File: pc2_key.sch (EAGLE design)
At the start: 25 parts, among them IC1 4011D, IC2 MC34063AD

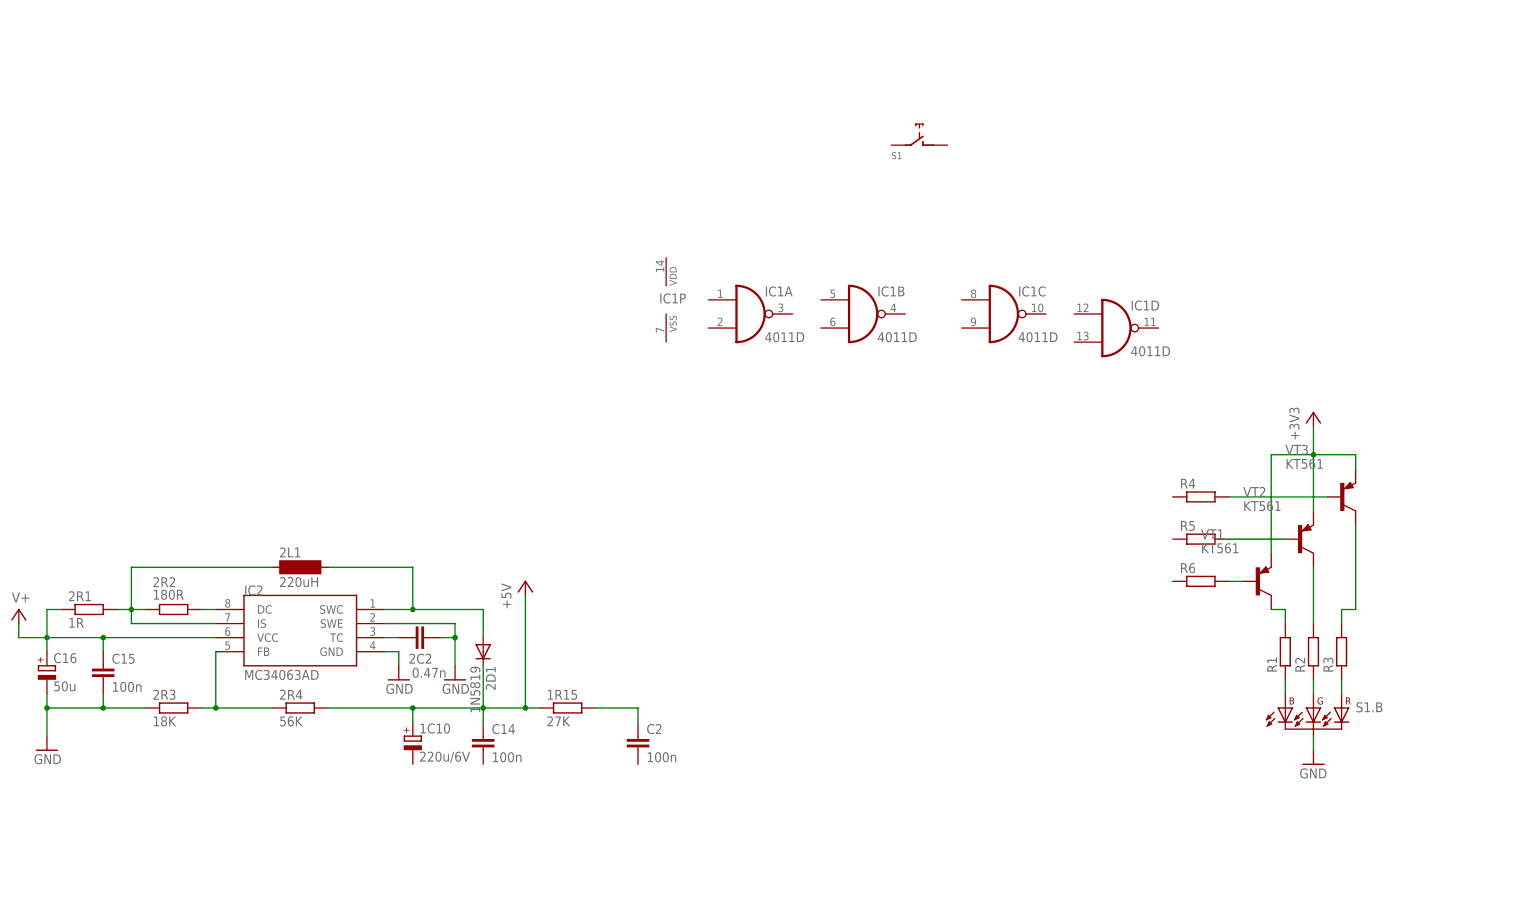
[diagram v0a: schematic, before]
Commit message: 2
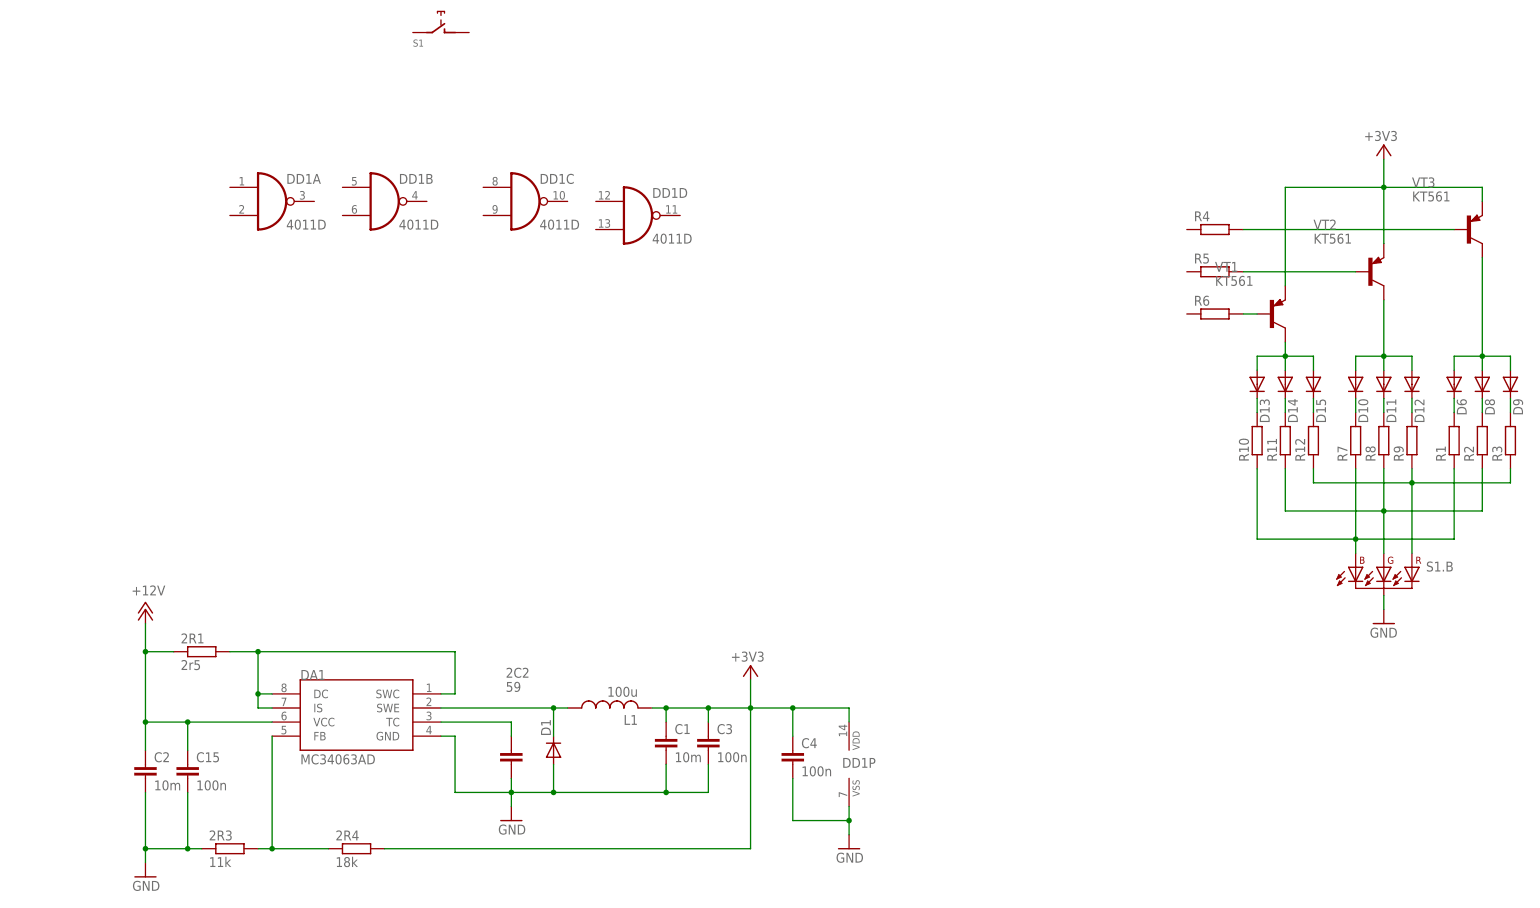
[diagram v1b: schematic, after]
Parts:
- removed 1C10: 220u/6V, resistor:CPOL-EUE3.5-8
- removed 1R15: 27K, resistor:R-EU_R0805
- removed 2D1: 1N5819, diode:DIODE-DO41-10
- removed 2L1: 220uH, inductor-neosid:SD12-1000
- removed 2R2: 180R, resistor:R-EU_R0805
- removed C14: 100n, resistor:C-EUC0805K
- removed C16: 50u, resistor:CPOL-EUE2.5-6
- removed IC1: 4011D, 40xx:4011D
- removed IC2: MC34063AD, mc34063:MC34063AD
- added C1: 10m, rcl:C-EUC1210
- added C3, C4: 100n, resistor:C-EUC0805K
- added D1: (no value), diode:DIODE-SMB
- added D10, D11, D12, D13, D14, D15, D6, D8, D9: (no value), diode:DIODE-SOD80C
- added DA1: MC34063AD, mc34063:MC34063AD
- added DD1: 4011D, 40xx:4011D
- added L1: 100u, rcl:L-US6000-XXX-RC
- added R10, R11, R12, R7, R8, R9: (no value), rcl:R-EU_R0805
- 2C2: value 0.47n -> 59
- 2R1: value 1R -> 2r5
- 2R3: value 18K -> 11k
- 2R4: value 56K -> 18k
- C2: value 100n -> 10m; device resistor:C-EUC0805K -> rcl:C-EUC1210
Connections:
- removed net +5V: 1C10.+, 1R15.1, 2D1.C, 2R4.2, C14.1
- removed net N$11: 1R15.2, C2.1
- removed net N$21: 2D1.A, 2L1.2, IC2.SWC
- removed net N$22: 2R2.2, IC2.DC
- removed net N$24: 2L1.1, 2R1.2, 2R2.1, IC2.IS
- removed net V+: 2R1.1, C15.1, C16.+, IC2.VCC
- new net +12V: 2R1.1, C15.1, C2.1, DA1.VCC
- new net N$13: R11.1, R2.1, R8.1, S1.B.G
- new net N$14: R12.1, R3.1, R9.1, S1.B.R
- new net N$15: D12.C, R9.2
- new net N$16: D11.C, R8.2
- new net N$17: D10.C, R7.2
- new net N$18: D15.C, R12.2
- new net N$20: D14.C, R11.2
- new net N$23: D13.C, R10.2
- new net N$26: D13.A, D14.A, D15.A, VT1.C
- new net N$27: D10.A, D11.A, D12.A, VT2.C
- new net N$28: D6.A, D8.A, D9.A, VT3.C
- net +3V3: now also 2R4.2, C1.1, C3.1, C4.1, DD1P.VDD, L1.2
- net GND: now also C1.2, C2.2, C3.2, C4.2, D1.A, DA1.GND, DD1P.VSS; no longer C16.-, IC2.GND, IC2.SWE
- net N$19: now also D1.C, DA1.SWE, L1.1; no longer 2C2.1, IC2.TC
- net N$25: now also DA1.FB; no longer IC2.FB
- net N$3: now also 2R1.2, DA1.DC, DA1.IS, DA1.SWC; no longer R1.2, VT1.C
- net N$4: now also R1.1, R10.1, R7.1, S1.B.B; no longer R2.2, VT2.C
- net N$5: now also 2C2.1, DA1.TC; no longer R3.2, VT3.C
- net N$6: now also D9.C, R3.2; no longer R1.1, S1.B.B
- net N$7: now also D8.C, R2.2; no longer R2.1, S1.B.G
- net N$8: now also D6.C, R1.2; no longer R3.1, S1.B.R
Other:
- moved on the sheet: 2C2, 2R1, 2R3, 2R4, C15, C2, R1, R2, R3, R4, R5, R6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
